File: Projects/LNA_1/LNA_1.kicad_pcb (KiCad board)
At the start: 2 copper layers, 59.7 x 41.9 mm, 31 parts, among them J1 SMA-J-P-H-ST-EM1, J2 SMA-J-P-H-ST-EM1, J3 Barrel_Jack_MountingPin, Q1 Q_NPN_BEC, U1 BFU790F

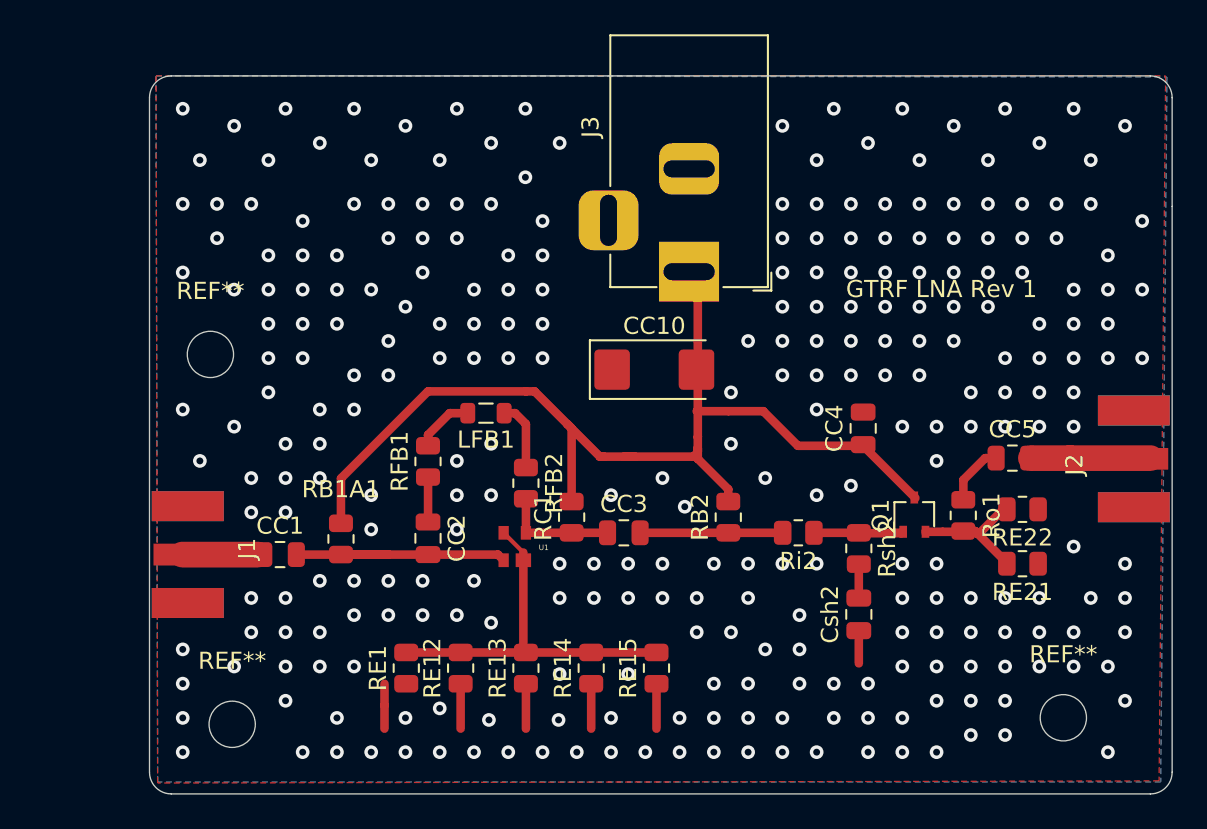
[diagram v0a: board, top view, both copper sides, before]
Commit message: last update
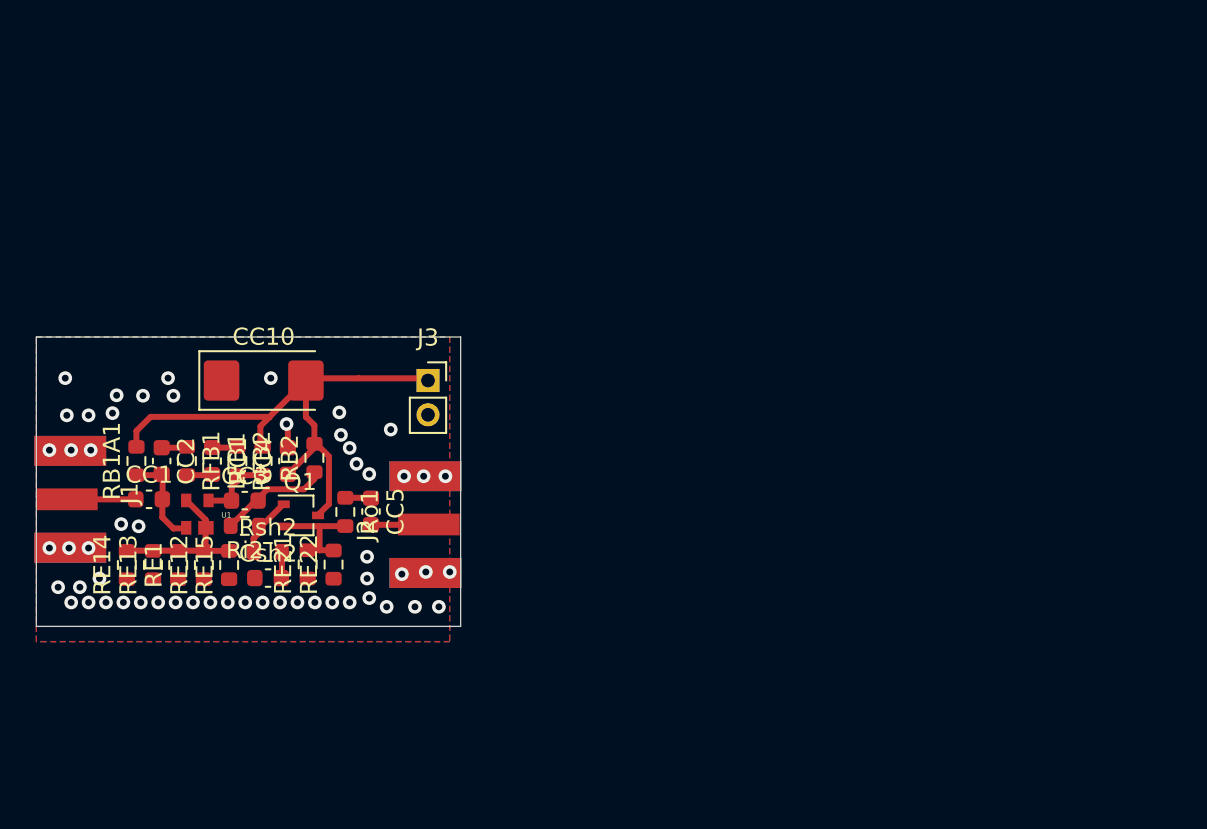
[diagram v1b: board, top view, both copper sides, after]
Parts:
- removed REF** (x3): MountingHole_2.7mm_M2.5, MountingHole:MountingHole_2.7mm_M2.5
- CC1, CC2, CC3, CC4, CC5, Csh2: footprint Capacitor_SMD:C_0805_2012Metric -> Capacitor_SMD:C_0603_1608Metric
- J1, J2: footprint AdditionalLibs:SAMTEC_SMA-J-P-H-ST-EM1 -> SAMTEC_SMA-J-P-H-ST-EM1
- J3: value Barrel_Jack_MountingPin -> Conn_01x02; footprint Connector_BarrelJack:BarrelJack_Horizontal -> Connector_PinSocket_2.00mm:PinSocket_1x02_P2.00mm_Vertical
- LFB1: footprint Inductor_SMD:L_0805_2012Metric -> Inductor_SMD:L_0603_1608Metric
- RB1A1, RB2, RC1, RE1, RE12, RE13, RE14, RE15, RE21, RE22, RFB1, RFB2, Ri2, Ro1, Rsh2: footprint Resistor_SMD:R_0805_2012Metric -> Resistor_SMD:R_0603_1608Metric
- moved RE21 41.7 mm to (120.0, 67.9), turned to 90 degrees
- moved J2 41.5 mm to (127.1, 65.6)
- moved RE22 40.3 mm to (121.5, 67.9), turned to 90 degrees
- moved CC5 37.6 mm to (123.7, 64.8), turned to 270 degrees
- moved Ro1 36.1 mm to (122.2, 64.8)
- moved Q1 35.8 mm to (119.6, 65.0), turned to 0 degrees
- moved Csh2 34.5 mm to (117.7, 68.7), turned to 0 degrees
- moved Rsh2 34.5 mm to (117.7, 67.2), turned to 0 degrees
- moved CC4 33.6 mm to (118.8, 61.8)
- moved Ri2 32.3 mm to (116.3, 65.6)
- moved RE14 27.8 mm to (109.4, 67.9)
- moved RE15 25.7 mm to (115.4, 67.9)
- moved RB2 24.4 mm to (120.4, 61.7)
- moved CC10 22.8 mm to (117.4, 57.1)
- moved RE13 22.6 mm to (110.9, 67.9)
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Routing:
- net VCC: track 61.5 -> 32.3 mm
- net GND: track 15.0 -> 1.42 mm, vias 287 -> 56
- net Net-(RE1-Pad2): track 22.1 -> 9.56 mm
- net Net-(CC1-Pad2): track 15.0 -> 5.75 mm
- net Net-(Q1-Pad1): track 7.73 -> 3.74 mm
- net Net-(CC5-Pad2): track 6.99 -> 3.19 mm
- net Net-(LFB1-Pad1): track 4.07 -> 1.55 mm
- net Net-(CC3-Pad1): track 6.81 -> 4.48 mm
- net Net-(LFB1-Pad2): track 3.48 -> 1.44 mm
- net Net-(CC5-Pad1): track 3.30 -> 1.54 mm
- net Net-(CC3-Pad2): track 8.13 -> 6.52 mm
- net Net-(CC2-Pad1): track 2.62 -> 1.56 mm
- net Net-(Q1-Pad2): track 7.71 -> 6.66 mm
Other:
- board size 59.7 x 41.9 mm -> 24.8 x 16.9 mm
- board text removed: "GTRF LNA Rev 1"
